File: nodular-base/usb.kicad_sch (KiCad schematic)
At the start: 7 parts, among them J7 USB_C_Receptacle_USB2.0, J8 USB_C_Receptacle_USB2.0, U2 FUSB302BMPX, U3 BQ25895RTW

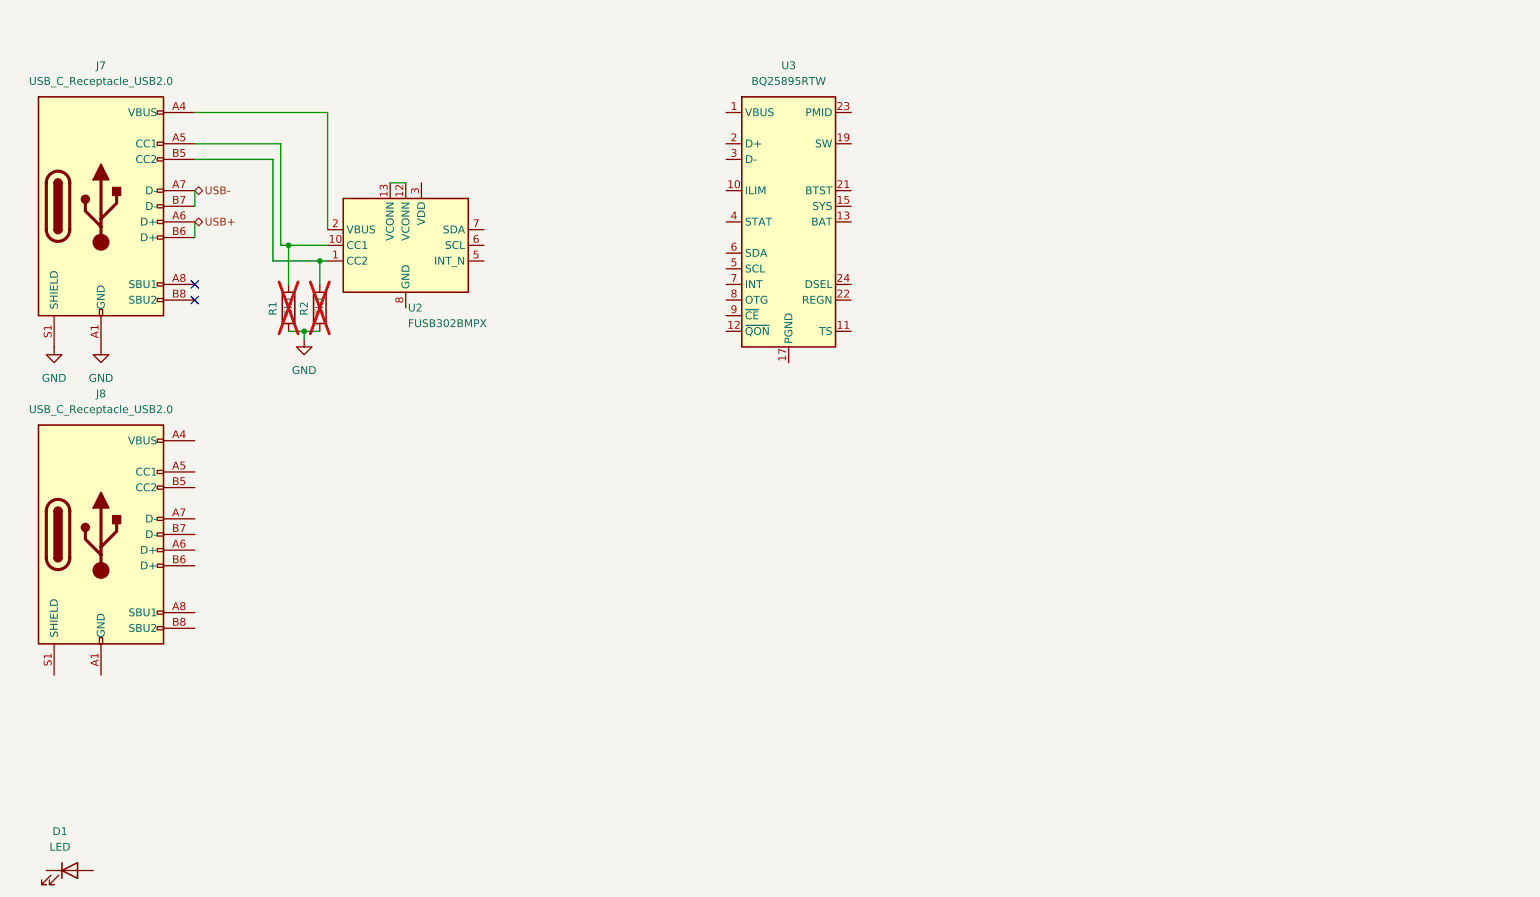
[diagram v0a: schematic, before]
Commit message: WIP layout for base
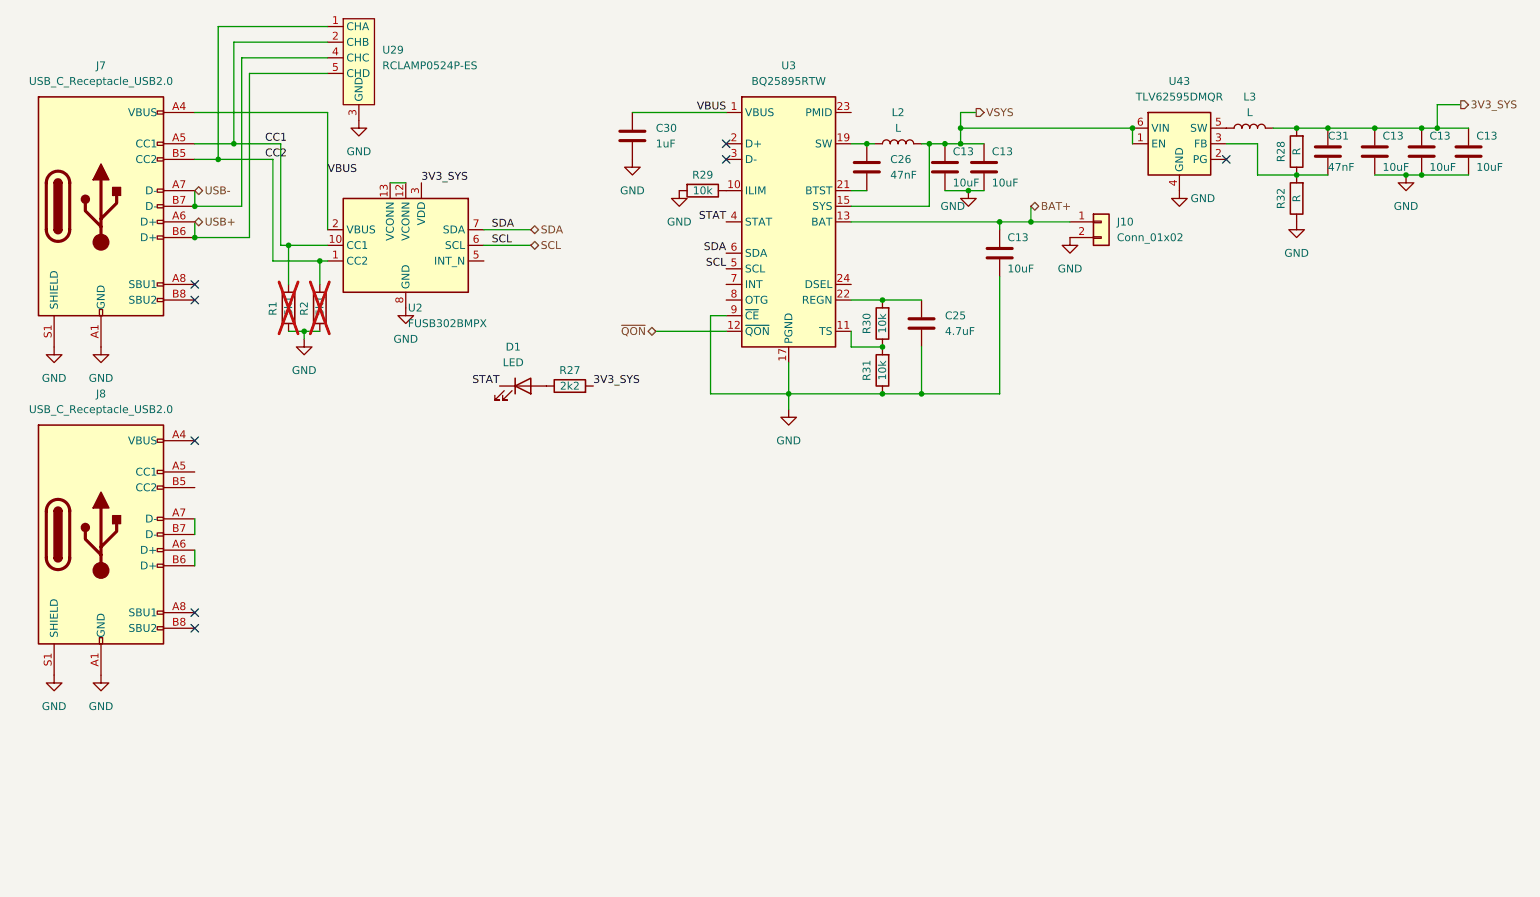
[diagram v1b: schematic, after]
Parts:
- added C13 (x6): 10uF, Capacitor_SMD:C_1206_3216Metric, symbol Device:C
- added C25: 4.7uF, Capacitor_SMD:C_0603_1608Metric, symbol Device:C
- added C26, C31: 47nF, Capacitor_SMD:C_0402_1005Metric, symbol Device:C
- added C30: 1uF, Capacitor_SMD:C_0603_1608Metric, symbol Device:C
- added J10: Conn_01x02, JST_PH_B2B-PH-SM4-TB_1x02-1MP_P2.00mm_Vertical, symbol Connector_Generic:Conn_01x02
- added L2: L, Inductor_SMD_Wurth:L_Wurth_WE-LQSH-4020, symbol Device:L
- added L3: L, Inductor_SMD_Wurth:L_Wurth_WE-LQSH-2512, symbol Device:L
- added R27: 2k2, Resistor_SMD:R_0402_1005Metric, symbol Device:R
- added R28, R32: R, Resistor_SMD:R_0402_1005Metric, symbol Device:R
- added R29, R30, R31: 10k, Resistor_SMD:R_0402_1005Metric, symbol Device:R
- added U29: RCLAMP0524P-ES, Package_DFN_QFN:Diodes_UDFN-10_1.0x2.5mm_P0.5mm, symbol nodular:RCLAMP0524P-ES
- added U43: TLV62595DMQR, nodular:Texas_VSON-HR-6_1.5x1.5mm_P0.5mm, symbol nodular:TLV62595DMQR
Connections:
- net GND: now also J8.A1 (GND), J8.A12 (GND), J8.B1 (GND), J8.B12 (GND), J8.S1 (SHIELD), U2.15 (GND), U2.8 (GND), U2.9 (GND), U3.17 (PGND), U3.18 (PGND), U3.25 (PGND), U3.9 (~{CE}), C13.2, C13.2, C13.2, C13.2, C13.2, C13.2, C25.2, C30.2, J10.2 (Pin_2), R29.2, R31.1, R32.1, U29.3 (GND), U29.8 (GND), U43.4 (GND)
- net USB+: now also U29.5 (CHD), U29.6 (CHD)
- net USB-: now also U29.4 (CHC), U29.7 (CHC)
- net STAT: now reaches D1.1 (K)
- net STAT: now also U3.4 (STAT)
- net at D1.2 (A): now also R27.1
- net VBUS: now reaches J7.A4 (VBUS), J7.A9 (VBUS), J7.B4 (VBUS), J7.B9 (VBUS), U2.2 (VBUS)
- net VBUS: now also U3.1 (VBUS), C30.1
- net CC1: now reaches J7.A5 (CC1), R1.1, U2.10 (CC1), U2.11 (CC1)
- net CC1: now also U29.2 (CHB), U29.9 (CHB)
- net CC2: now reaches J7.B5 (CC2), R2.1, U2.1 (CC2), U2.14 (CC2)
- net CC2: now also U29.1 (CHA), U29.10 (CHA)
- net at J8.A6 (D+): now also J8.B6 (D+)
- net at J8.A7 (D-): now also J8.B7 (D-)
- net 3V3_SYS: now reaches U2.3 (VDD), U2.4 (VDD)
- net 3V3_SYS: now also C13.1, C13.1, C13.1, C31.1, L3.2, R27.2, R28.2
- net SCL: now reaches U2.6 (SCL)
- net SCL: now also U3.5 (SCL)
- net SDA: now reaches U2.7 (SDA)
- net SDA: now also U3.6 (SDA)
- net at U3.10 (ILIM): now also R29.1
- net at U3.11 (TS): now also R30.1, R31.2
- net ~{QON}: now reaches U3.12 (~{QON})
- net BAT+: now reaches U3.13 (BAT), U3.14 (BAT)
- net BAT+: now also C13.1, J10.1 (Pin_1)
- net VSYS: now reaches U3.15 (SYS), U3.16 (SYS)
- net VSYS: now also C13.1, C13.1, L2.2, U43.1 (EN), U43.6 (VIN)
- net at U3.19 (SW), U3.20 (SW): now also C26.1, L2.1
- net at U3.21 (BTST): now also C26.2
- net at U3.22 (REGN): now also C25.1, R30.2
- new net: C31.2, R28.1, R32.2, U43.3 (FB)
- new net: L3.1, U43.5 (SW)
- no-connect marks 2 -> 8
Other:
- moved on the sheet: D1
